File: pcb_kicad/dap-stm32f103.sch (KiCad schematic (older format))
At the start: 35 parts, among them J1 USB_C_Receptacle_USB2.0, J2 Conn_01x10, J3 Conn_01x10, J4 Conn_01x10, U1 STM32F103CBTx, Y1 SMD-5032_2P_8MHz_20ppm_20pF

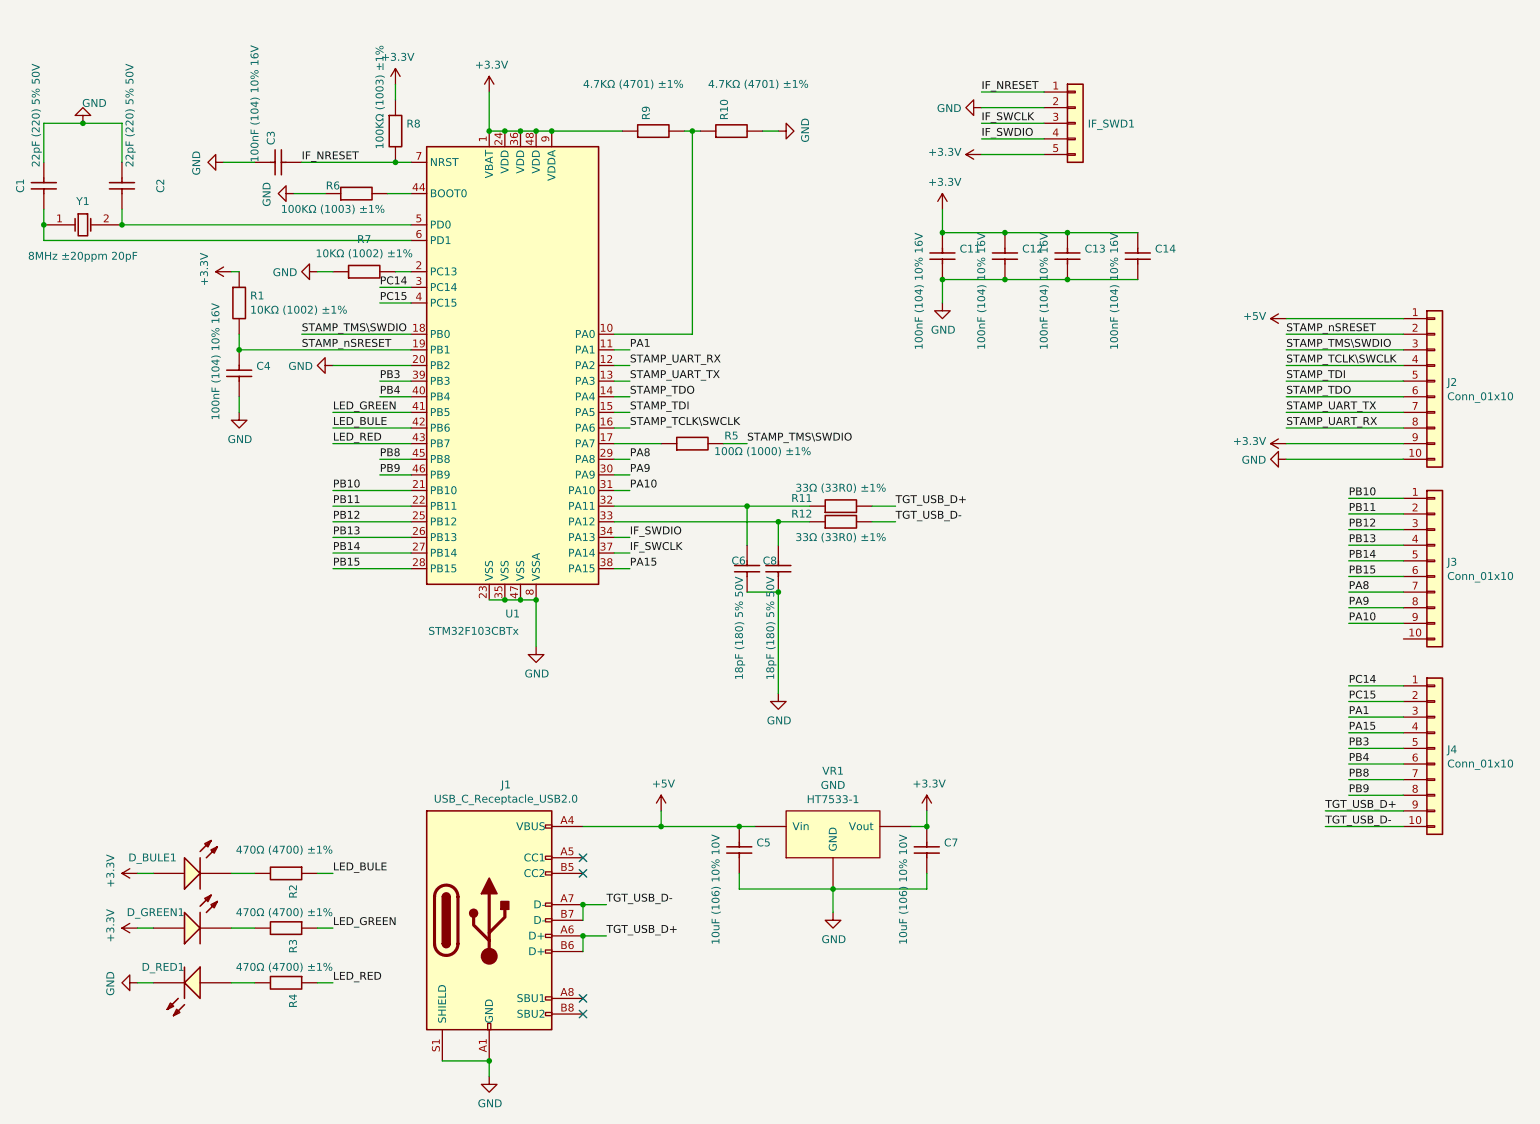
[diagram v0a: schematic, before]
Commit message: [done] stamp pcb
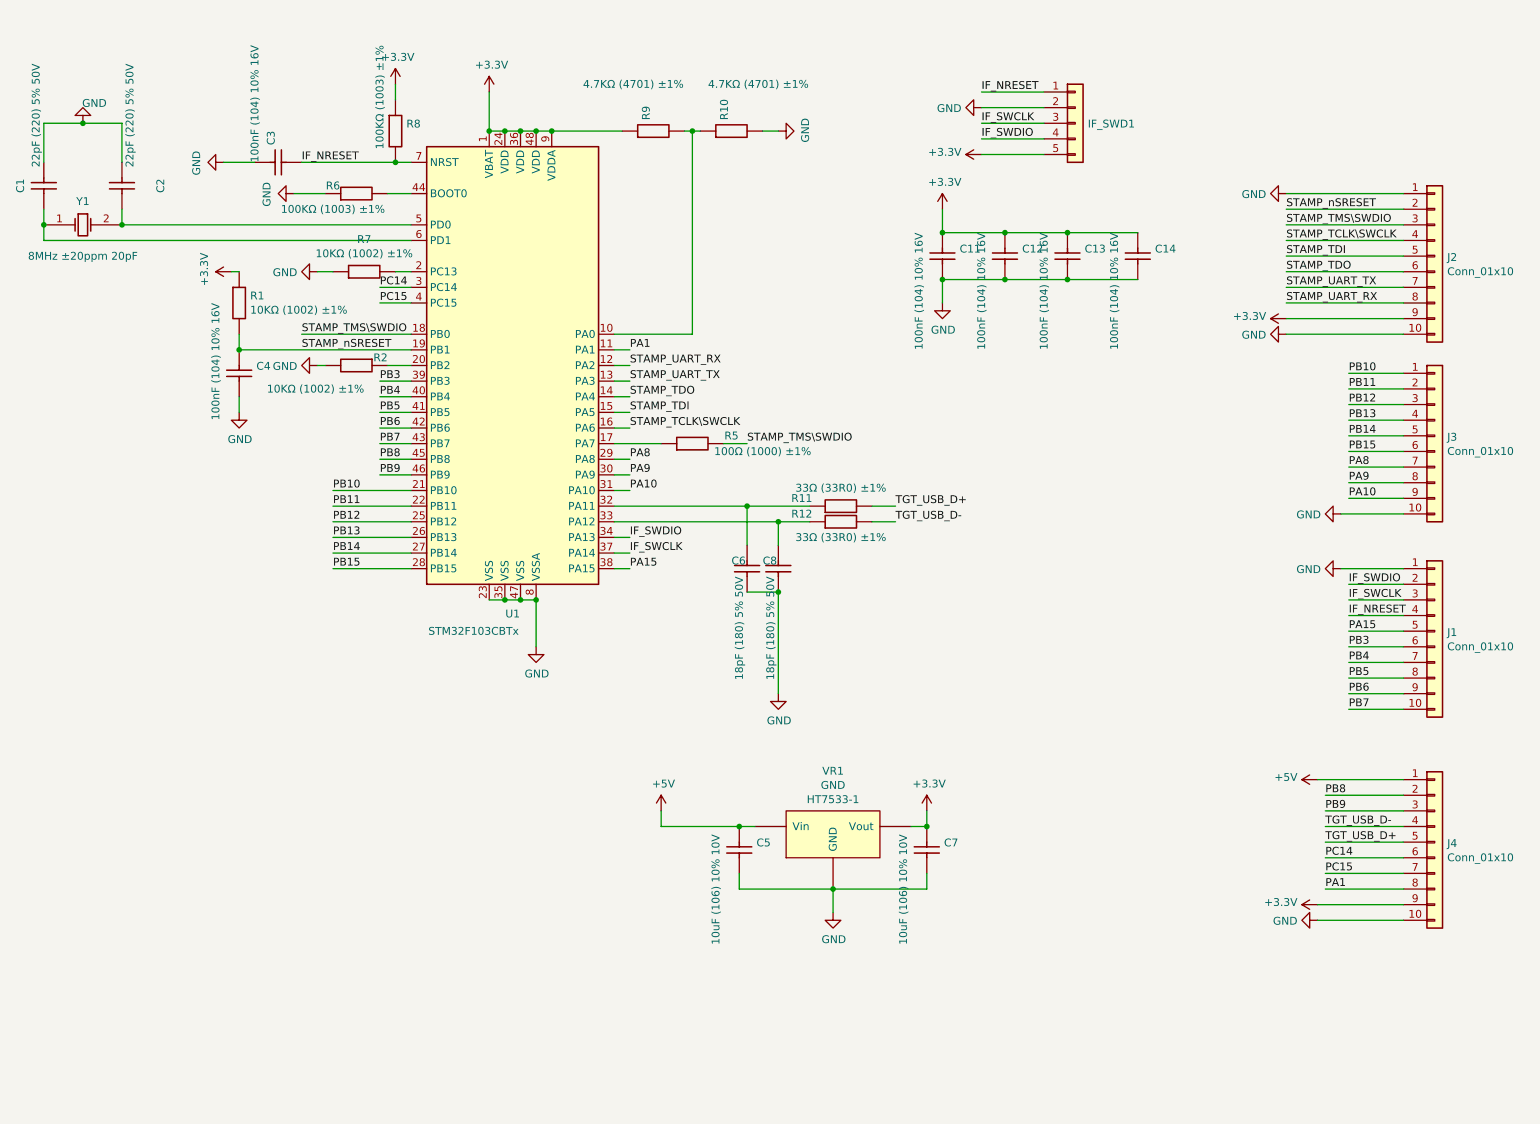
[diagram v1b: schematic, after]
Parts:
- removed D_BULE1: 0603_蓝灯, lc_lib:0603_LED_S1, symbol lc_LED:0603_蓝灯
- removed D_GREEN1: 0603_绿灯, lc_lib:0603_LED_S1, symbol lc_LED:0603_绿灯
- removed D_RED1: 0603_红灯, lc_lib:0603_LED_S1, symbol lc_LED:0603_红灯
- removed J1: USB_C_Receptacle_USB2.0, Connector_USB:USB_C_Receptacle_Palconn_UTC16-G, symbol Connector:USB_C_Receptacle_USB2.0
- removed R2, R3, R4: 0402_470Ω__4700_1%, lc_lib:0402_R, symbol lc_RES:0402_470Ω__4700_1%
- added J1: Conn_01x10, lc_lib:stamp_2.0mm_1x10, symbol Connector_Generic:Conn_01x10
- added R2: 0402_10KΩ__1002_1%, lc_lib:0402_R, symbol lc_RES:0402_10KΩ__1002_1%
- IF_SWD1: footprint Connector_PinHeader_2.54mm:PinHeader_1x05_P2.54mm_Vertical -> Connector_PinSocket_1.27mm:PinSocket_1x05_P1.27mm_Vertical
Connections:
- net +3V3: now also J4.9 (Pin_9)
- net +5V: now also J4.1 (Pin_1); no longer J2.1 (Pin_1)
- net GND: now also J2.1 (Pin_1), J3.10 (Pin_10), J4.10 (Pin_10), J1.1 (Pin_1), R2.2; no longer U1.20 (PB2)
- net IF_NRESET: now also J1.4 (Pin_4)
- net IF_SWCLK: now also J1.3 (Pin_3)
- net IF_SWDIO: now also J1.2 (Pin_2)
- net PA1: now also J4.8 (Pin_8); no longer J4.3 (Pin_3)
- net PA15: now also J1.5 (Pin_5); no longer J4.4 (Pin_4)
- net PB3: now also J1.6 (Pin_6); no longer J4.5 (Pin_5)
- net PB4: now also J1.7 (Pin_7); no longer J4.6 (Pin_6)
- net PB8: now also J4.2 (Pin_2); no longer J4.7 (Pin_7)
- net PB9: now also J4.3 (Pin_3); no longer J4.8 (Pin_8)
- net PC14: now also J4.6 (Pin_6); no longer J4.1 (Pin_1)
- net PC15: now also J4.7 (Pin_7); no longer J4.2 (Pin_2)
- net TGT_USB_D+: now also J4.5 (Pin_5); no longer J4.9 (Pin_9)
- net TGT_USB_D-: now also J4.4 (Pin_4); no longer J4.10 (Pin_10)
- net LED_BULE renamed PB6
- net PB6: now also J1.9 (Pin_9)
- net LED_GREEN renamed PB5
- net PB5: now also J1.8 (Pin_8)
- net LED_RED renamed PB7
- net PB7: now also J1.10 (Pin_10)
- new net: R2.1, U1.20 (PB2)
- no-connect marks 4 -> 0
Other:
- moved on the sheet: J2, J3, J4
